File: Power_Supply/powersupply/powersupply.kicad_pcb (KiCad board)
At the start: 2 copper layers, 62.2 x 0.2 mm, 65 parts, among them J1 Conn_01x03, J2 USB_B_Micro, Q1 Q_PMOS_GDS, SW1 SW_Push, U1 AZ1117E-3.3, U10 MCP6001-OT, U2 ATSAMD10D13A-SS, U3 B0505S-2WR2, U4 TFT_OLED, U5 joystick-K1-1506DN-01, U6 MC33063AP1, U7 LM358P, U8 1x2, U9 1x2

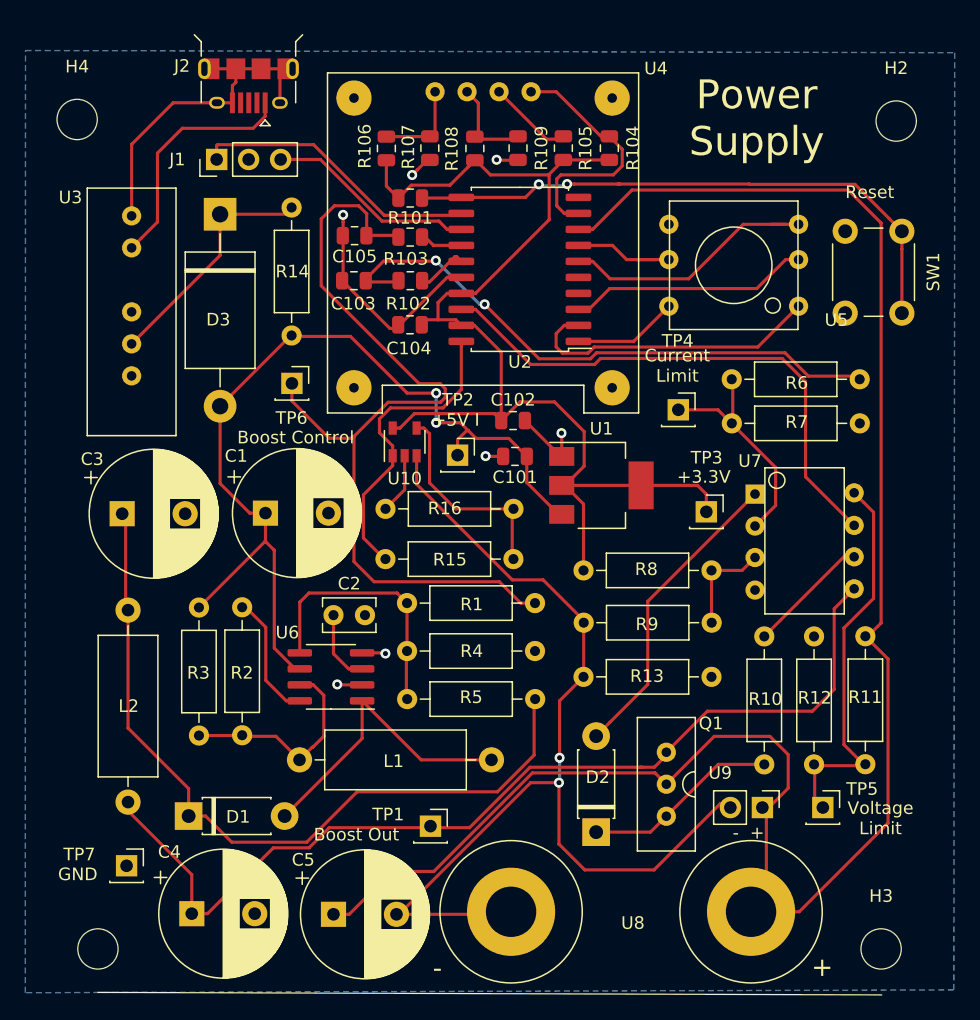
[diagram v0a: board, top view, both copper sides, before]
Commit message: check
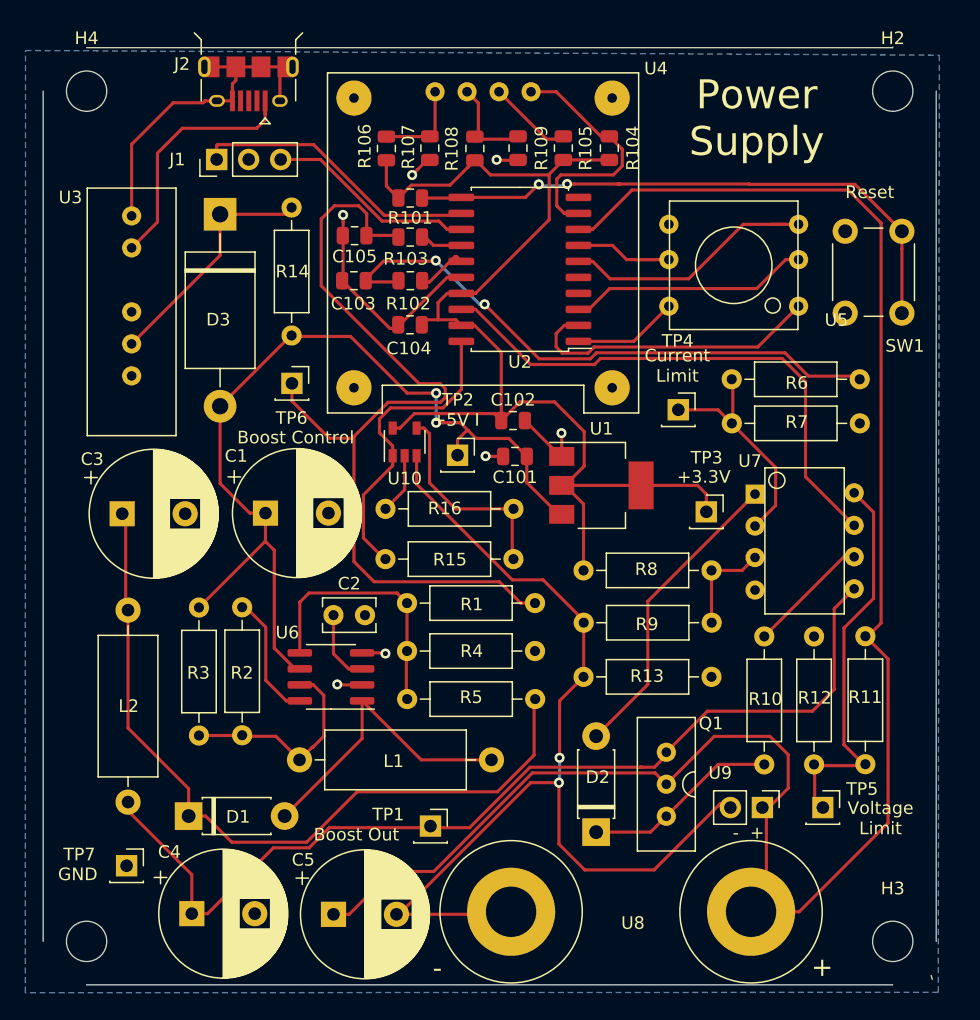
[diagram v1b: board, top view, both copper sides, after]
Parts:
- moved H2 2.39 mm to (114.0, 22.5)
- moved H4 2.37 mm to (50.0, 22.5)
- moved H3 1.10 mm to (114.0, 90.0)
- moved H1 1.08 mm to (50.0, 90.0)
- moved J2 0.15 mm to (62.9, 20.6)
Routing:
- net Net-(J2-Pad1): track 19.2 -> 20.6 mm
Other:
- board size 62.2 x 0.2 mm -> 70.9 x 74.5 mm
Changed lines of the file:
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@@
   (general
     (thickness 1.6)
-    (drawings 13)
-    (tracks 417)
+    (drawings 18)
+    (tracks 419)
     (zones 0)
     (modules 65)
@@
     (mod_text_size 1 1)
     (mod_text_width 0.15)
-    (pad_size 1.524 1.524)
-    (pad_drill 0.762)
+    (pad_size 3.2 3.2)
+    (pad_drill 3.2)
     (pad_to_mask_clearance 0.051)
     (solder_mask_min_width 0.25)
@@
   )
   (module MountingHole:MountingHole_3.2mm_M3 (layer F.Cu)
-    (at 49.25 24.75)
+    (at 50 22.5)
     (descr "Mounting Hole 3.2mm, no annular, M3")
     (tags "mounting hole 3.2mm no annular m3")
@@
   )
   (module MountingHole:MountingHole_3.2mm_M3 (layer F.Cu)
-    (at 113.075 90.6)
+    (at 114 90)
     (descr "Mounting Hole 3.2mm, no annular, M3")
     (tags "mounting hole 3.2mm no annular m3")
@@
   )
   (module MountingHole:MountingHole_3.2mm_M3 (layer F.Cu)
-    (at 114.275 24.875)
+    (at 114 22.5)
     (descr "Mounting Hole 3.2mm, no annular, M3")
     (tags "mounting hole 3.2mm no annular m3")
@@
   )
   (module MountingHole:MountingHole_3.2mm_M3 (layer F.Cu)
-    (at 50.9 90.6)
+    (at 50 90)
     (descr "Mounting Hole 3.2mm, no annular, M3")
     (tags "mounting hole 3.2mm no annular m3")
@@
     (descr https://www.omron.com/ecb/products/pdf/en-b3f.pdf)
     (tags "tact sw push 6mm")
-    (fp_text reference SW1 (at 3.2232 -2.4986 90) (layer F.SilkS)
+    (fp_text reference SW1 (at 9.0978 -0.2354 180) (layer F.SilkS)
       (effects (font (size 1 1) (thickness 0.15)))
     )
@@
   )
   (module powersupply:USB_Micro-B_Amphenol_10118194-0001LF_Horizontal (layer F.Cu)
-    (at 62.85 20.725 180)
+    (at 62.85 20.5726 180)
     (tags "USB USB_B USB_micro USB_OTG")
     (attr smd)
@@
     )
   )
-  (gr_line (start 113.125 94.25) (end 50.9 94.05) (layer Edge.Cuts) (width 0.05))
+  (gr_line (start 113.9952 19.05) (end 113.9952 18.9992) (layer Edge.Cuts) (width 0.05))
+  (gr_line (start 50 19.05) (end 114 19.05) (layer Edge.Cuts) (width 0.05))
+  (gr_line (start 46.55 22.5) (end 46.55 90) (layer Edge.Cuts) (width 0.05))
+  (gr_line (start 117.1448 93.0148) (end 117.0432 92.71) (layer Edge.Cuts) (width 0.05))
+  (gr_line (start 117.45 22.5) (end 117.45 90) (layer Edge.Cuts) (width 0.05))
+  (gr_line (start 114 93.45) (end 50 93.45) (layer Edge.Cuts) (width 0.05))
   (gr_text "Power\nSupply" (at 103.2 24.65) (layer F.SilkS)
     (effects (font (size 2.3 2.3) (thickness 0.3)))
@@
   (segment (start 79.5954 32.3596) (end 73.63242 32.3596) (width 0.25) (layer F.Cu) (net 15))
   (segment (start 79.75 32.205) (end 79.5954 32.3596) (width 0.25) (layer F.Cu) (net 15))
-  (segment (start 59.95 20.725) (end 65.75 20.725) (width 0.25) (layer F.Cu) (net 16))
-  (segment (start 61.575 22.35) (end 61.575 23.425) (width 0.25) (layer F.Cu) (net 16))
-  (segment (start 61.575 22.075) (end 61.575 22.35) (width 0.25) (layer F.Cu) (net 16))
-  (segment (start 61.85 21.8) (end 61.575 22.075) (width 0.25) (layer F.Cu) (net 16))
-  (segment (start 61.85 20.725) (end 61.85 21.8) (width 0.25) (layer F.Cu) (net 16))
-  (segment (start 61.575 23.425) (end 60.35 23.425) (width 0.25) (layer F.Cu) (net 16))
-  (segment (start 65.35 21.125) (end 65.75 20.725) (width 0.25) (layer F.Cu) (net 16))
-  (segment (start 65.35 23.425) (end 65.35 21.125) (width 0.25) (layer F.Cu) (net 16))
-  (segment (start 60.35 23.425) (end 60.2 23.425) (width 0.25) (layer F.Cu) (net 16))
-  (segment (start 56.875 23.425) (end 60.35 23.425) (width 0.25) (layer F.Cu) (net 16))
+  (segment (start 59.95 20.5726) (end 65.75 20.5726) (width 0.25) (layer F.Cu) (net 16))
+  (segment (start 61.575 22.1976) (end 61.575 23.2726) (width 0.25) (layer F.Cu) (net 16))
+  (segment (start 61.575 21.9226) (end 61.575 22.1976) (width 0.25) (layer F.Cu) (net 16))
+  (segment (start 61.85 21.6476) (end 61.575 21.9226) (width 0.25) (layer F.Cu) (net 16))
+  (segment (start 61.85 20.5726) (end 61.85 21.6476) (width 0.25) (layer F.Cu) (net 16))
+  (segment (start 61.575 23.2726) (end 60.35 23.2726) (width 0.25) (layer F.Cu) (net 16))
+  (segment (start 65.35 20.9726) (end 65.75 20.5726) (width 0.25) (layer F.Cu) (net 16))
+  (segment (start 65.35 23.2726) (end 65.35 20.9726) (width 0.25) (layer F.Cu) (net 16))
+  (segment (start 60.35 23.2726) (end 60.2 23.2726) (width 0.25) (layer F.Cu) (net 16))
   (segment (start 53.575 26.725) (end 56.875 23.425) (width 0.25) (layer F.Cu) (net 16))
   (segment (start 53.575 32.405) (end 53.575 26.725) (width 0.25) (layer F.Cu) (net 16))
-  (segment (start 54.336999 34.183001) (end 53.575 34.945) (width 0.25) (layer F.Cu) (net 17))
-  (segment (start 55.625 32.895) (end 54.336999 34.183001) (width 0.25) (layer F.Cu) (net 17))
-  (segment (start 55.625 27.425) (end 55.625 32.895) (width 0.25) (layer F.Cu) (net 17))
-  (segment (start 63.225 25.45) (end 57.6 25.45) (width 0.25) (layer F.Cu) (net 17))
-  (segment (start 57.6 25.45) (end 55.625 27.425) (width 0.25) (layer F.Cu) (net 17))
-  (segment (start 64.175 24.5) (end 63.225 25.45) (width 0.25) (layer F.Cu) (net 17))
-  (segment (start 64.175 23.425) (end 64.175 24.5) (width 0.25) (layer F.Cu) (net 17))
+  (segment (start 59.239 23.425) (end 59.3914 23.2726) (width 0.25) (layer F.Cu) (net 16))
+  (segment (start 56.875 23.425) (end 59.239 23.425) (width 0.25) (layer F.Cu) (net 16))
+  (segment (start 59.3914 23.2726) (end 60.35 23.2726) (width 0.25) (layer F.Cu) (net 16))
+  (segment (start 64.175 23.2726) (end 64.175 24.3476) (width 0.25) (layer F.Cu) (net 17))
+  (segment (start 64.175 24.7758) (end 64.175 23.2726) (width 0.25) (layer F.Cu) (net 17))
+  (segment (start 63.5008 25.45) (end 64.175 24.7758) (width 0.25) (layer F.Cu) (net 17))
+  (segment (start 55.625 27.425) (end 57.6 25.45) (width 0.25) (layer F.Cu) (net 17))
+  (segment (start 55.625 32.895) (end 55.625 27.425) (width 0.25) (layer F.Cu) (net 17))
+  (segment (start 57.6 25.45) (end 63.5008 25.45) (width 0.25) (layer F.Cu) (net 17))
+  (segment (start 53.575 34.945) (end 55.625 32.895) (width 0.25) (layer F.Cu) (net 17))
   (segment (start 62.6612 73.6584) (end 62.7212 73.7184) (width 0.25) (layer F.Cu) (net 21))
   (segment (start 58.9212 73.6584) (end 62.6612 73.6584) (width 0.25) (layer F.Cu) (net 21))
@@
     (polygon
       (pts
-        (xy 45.15 19.275) (xy 118.925 19.45) (xy 118.85 93.85) (xy 45.125 94.075)
+        (xy 45.15 19.275) (xy 117.6903 19.6452) (xy 117.6153 94.0452) (xy 45.125 94.075)
       )
     )
